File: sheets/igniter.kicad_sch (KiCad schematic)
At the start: 18 parts, among them J18 Screw_Terminal_01x02, J19 Screw_Terminal_01x02, Q2 AO3400A, Q3 AO3400A

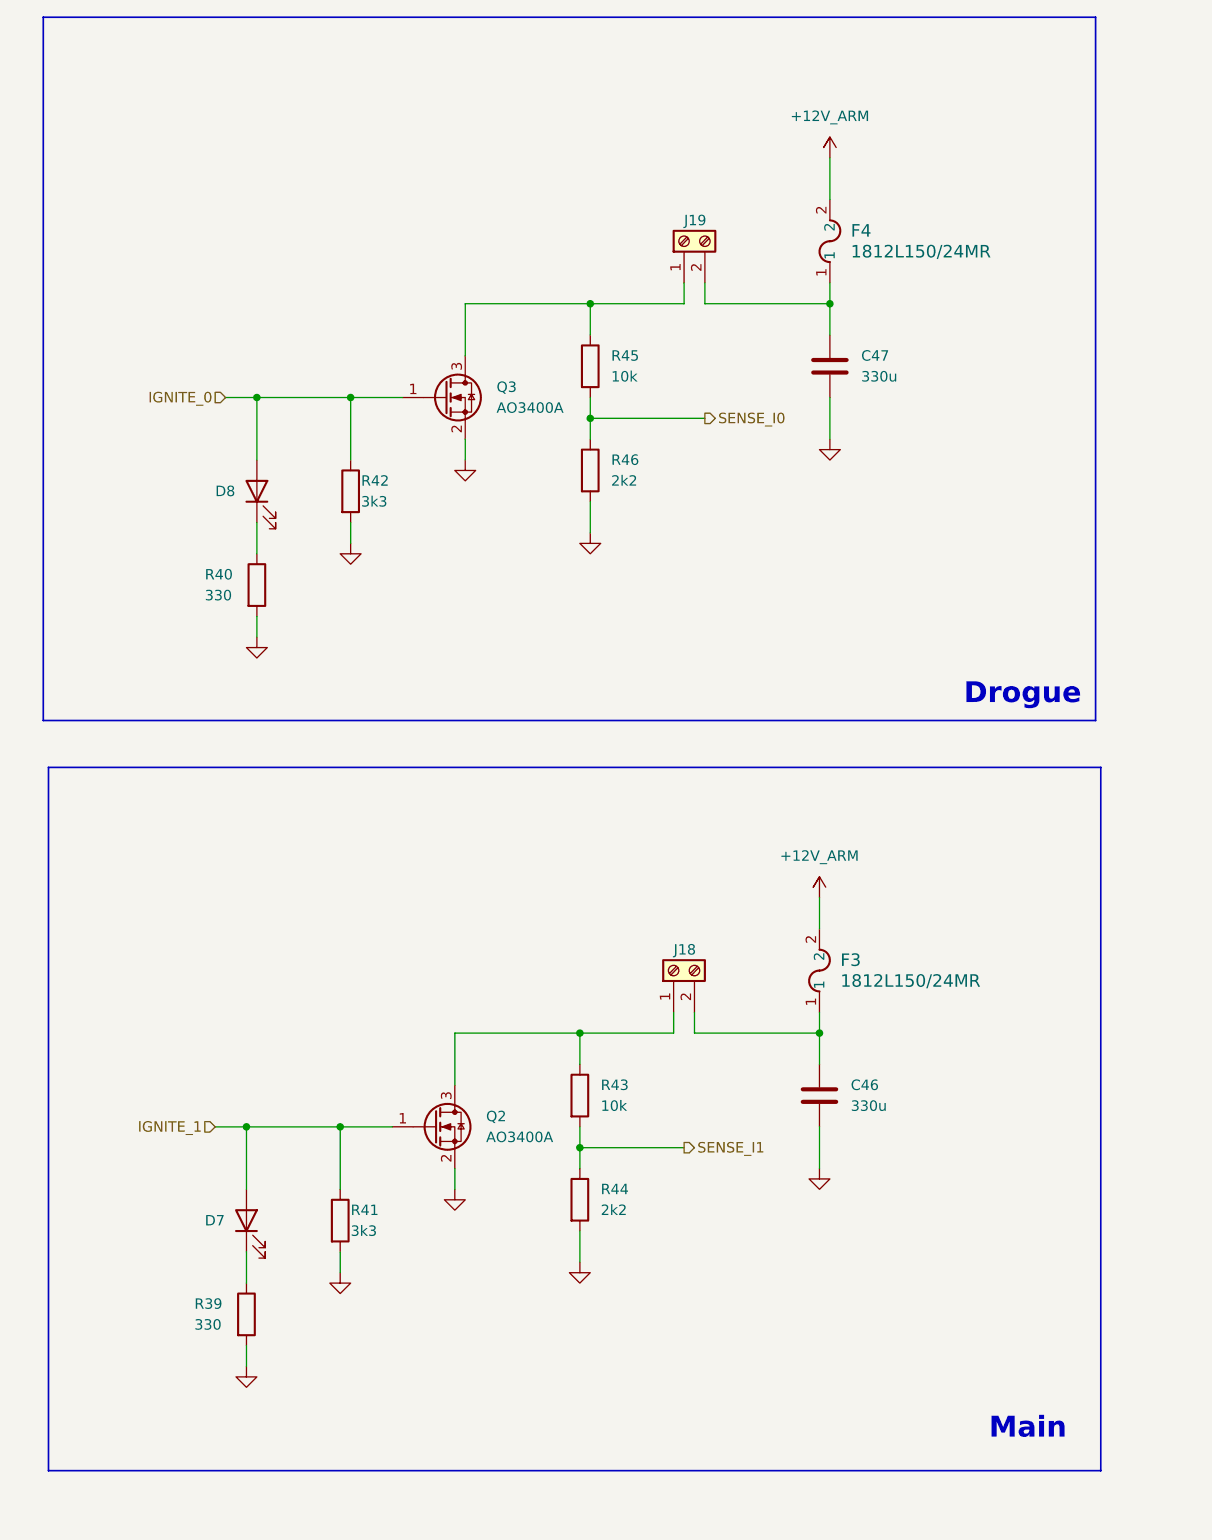
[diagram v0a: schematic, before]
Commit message: some changes for 2027 aerolotl
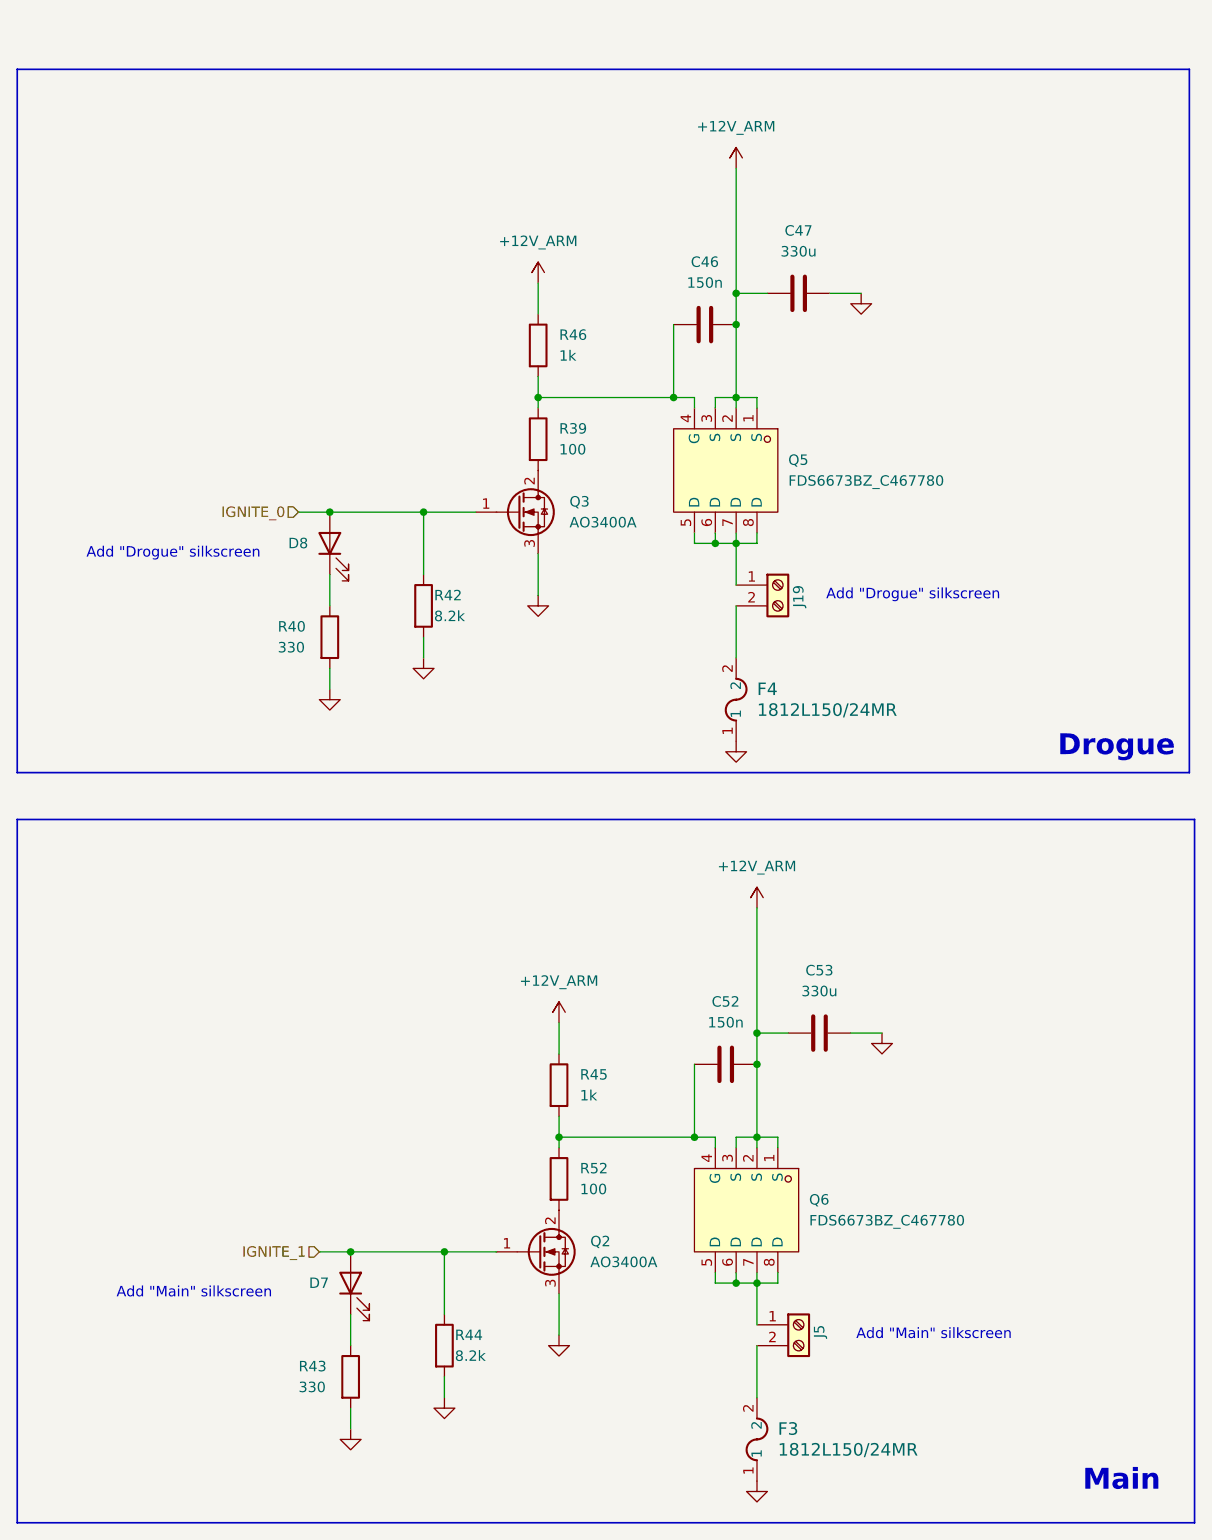
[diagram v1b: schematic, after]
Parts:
- removed J18: Screw_Terminal_01x02, symbol Connector:Screw_Terminal_01x02
- removed Q2, Q3: AO3400A, Package_TO_SOT_SMD:SOT-23, symbol Transistor_FET:AO3400A
- removed R41: 3k3, symbol Device:R
- added C52: 150n, symbol Device:C
- added C53: 330u, symbol Device:C
- added J5: Screw_Terminal_01x02, symbol Connector:Screw_Terminal_01x02
- added Q2, Q3: AO3400A, Package_TO_SOT_SMD:TO-252-2, symbol Transistor_FET:Q_NMOS_GDS
- added Q5, Q6: FDS6673BZ_C467780, aerolotl_custom:SOIC-8_L4.9-W3.9-P1.27-LS6.0-BL, symbol aerolotl_custom:FDS6673BZ_C467780
- added R52: 100, symbol Device:R
- C46: value 330u -> 150n
- R39: value 330 -> 100
- R42: value 3k3 -> 8.2k
- R43: value 10k -> 330
- R44: value 2k2 -> 8.2k
- R45: value 10k -> 1k
- R46: value 2k2 -> 1k
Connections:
- net +12V_ARM: now also C46.1, C47.2, R45.1, R46.1, C52.1, C53.2, Q5.1 (S), Q5.2 (S), Q5.3 (S), Q6.1 (S), Q6.2 (S), Q6.3 (S); no longer F3.2, F4.2
- net GND: now also C47.1, F3.1, F4.1, R43.2, C53.1, Q2.3 (S), Q3.3 (S); no longer C46.2, C47.2, R39.2, R46.2
- net IGNITE_0: now also Q3.1 (G)
- net IGNITE_1: now also R44.1, Q2.1 (G)
- net at J19.1 (Pin_1): now also Q5.5 (D), Q5.6 (D), Q5.7 (D), Q5.8 (D); no longer R45.1
- net at R39.1: now also C46.2, R46.2, Q5.4 (G); no longer D7.1 (K)
- net at R43.1: now also D7.1 (K)
- net SENSE_I0: no longer names the net of R45.2
- net SENSE_I0: now also C52.2, Q6.4 (G), R52.1; no longer R46.1
- removed net SENSE_I1: R43.2, R44.1
- new net: Q2.2 (D), R52.2
- new net: F4.2, J19.2 (Pin_2)
- new net: J5.1 (Pin_1), Q6.5 (D), Q6.6 (D), Q6.7 (D), Q6.8 (D)
- new net: F3.2, J5.2 (Pin_2)
- new net: Q3.2 (D), R39.2
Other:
- note added: "Add "Drogue" silkscreen"
- note added: "Add "Main" silkscreen"
- moved on the sheet: C47, D8, F4, J19, R40, R42, R46
